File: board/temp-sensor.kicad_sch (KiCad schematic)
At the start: 3 parts, among them J6 Conn_01x02

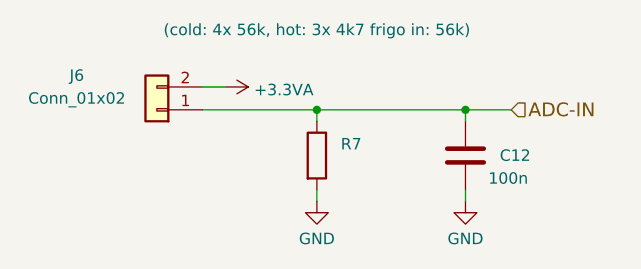
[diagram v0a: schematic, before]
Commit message: WIP
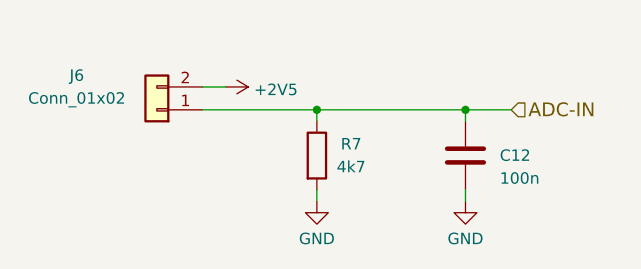
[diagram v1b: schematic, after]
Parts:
- R7: value (cold: 4x 56k, hot: 3x 4k7 frigo in: 56k) -> 4k7
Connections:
- net +3.3VA renamed +2V5
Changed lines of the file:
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@@
       (effects (font (size 1.27 1.27)))
     )
-    (property "Value" "(cold: 4x 56k, hot: 3x 4k7 frigo in: 56k)" (at 139.7 63.5 0)
+    (property "Value" "4k7" (at 143.51 78.74 0)
       (effects (font (size 1.27 1.27)))
     )
@@
       (effects (font (size 1.27 1.27)) (justify left))
     )
-    (property "Value" "100n" (at 158.75 80.01 0)
+    (property "Value" "100n" (at 160.02 80.01 0)
       (effects (font (size 1.27 1.27)) (justify left))
     )
@@
         (path "/bd0055da-0838-4c4c-b506-87ee1119a3e6/00000000-0000-0000-0000-00005c2319d5"
           (reference "C15") (unit 1)
+        )
+      )
+    )
+  )
+  (symbol (lib_id "power:+2V5") (at 129.54 69.85 270) (unit 1)
+    (in_bom yes) (on_board yes) (dnp no) (fields_autoplaced)
+    (property "Reference" "#PWR09" (at 125.73 69.85 0)
+      (effects (font (size 1.27 1.27)) hide)
+    )
+    (property "Value" "+2V5" (at 132.715 70.1668 90)
+      (effects (font (size 1.27 1.27)) (justify left))
+    )
+    (property "Footprint" "" (at 129.54 69.85 0)
+      (effects (font (size 1.27 1.27)) hide)
+    )
+    (property "Datasheet" "" (at 129.54 69.85 0)
+      (effects (font (size 1.27 1.27)) hide)
+    )
+    (pin "1")
+    (instances
+      (project "nanook-as"
+        (path "/bd0055da-0838-4c4c-b506-87ee1119a3e6/00000000-0000-0000-0000-00005c22fbc8"
+          (reference "#PWR09") (unit 1)
+        )
+        (path "/bd0055da-0838-4c4c-b506-87ee1119a3e6/00000000-0000-0000-0000-00005c23178f"
+          (reference "#PWR010") (unit 1)
+        )
+        (path "/bd0055da-0838-4c4c-b506-87ee1119a3e6/00000000-0000-0000-0000-00005c2318b8"
+          (reference "#PWR011") (unit 1)
+        )
+        (path "/bd0055da-0838-4c4c-b506-87ee1119a3e6/00000000-0000-0000-0000-00005c2319d5"
+          (reference "#PWR012") (unit 1)
         )
       )
@@
         )
       )
-    )
-  )
-  (symbol (lib_id "power:+3.3VA") (at 129.54 69.85 270) (unit 1)
-    (in_bom yes) (on_board yes) (dnp no) (fields_autoplaced)
-    (property "Reference" "#PWR0137" (at 125.73 69.85 0)
-      (effects (font (size 1.27 1.27)) hide)
-    )
-    (property "Value" "+3.3VA" (at 132.715 70.1819 90)
-      (effects (font (size 1.27 1.27)) (justify left))
-    )
-    (property "Footprint" "" (at 129.54 69.85 0)
-      (effects (font (size 1.27 1.27)) hide)
-    )
-    (property "Datasheet" "" (at 129.54 69.85 0)
-      (effects (font (size 1.27 1.27)) hide)
-    )
-    (pin "1")
-    (instances
-      (project "nanook-as"
-        (path "/bd0055da-0838-4c4c-b506-87ee1119a3e6/00000000-0000-0000-0000-00005c22fbc8"
-          (reference "#PWR0137") (unit 1)
-        )
-        (path "/bd0055da-0838-4c4c-b506-87ee1119a3e6/00000000-0000-0000-0000-00005c23178f"
-          (reference "#PWR0140") (unit 1)
-        )
-        (path "/bd0055da-0838-4c4c-b506-87ee1119a3e6/00000000-0000-0000-0000-00005c2318b8"
-          (reference "#PWR0143") (unit 1)
-        )
-        (path "/bd0055da-0838-4c4c-b506-87ee1119a3e6/00000000-0000-0000-0000-00005c2319d5"
-          (reference "#PWR0146") (unit 1)
-        )
-      )
